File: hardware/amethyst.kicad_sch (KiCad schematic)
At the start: 0 parts

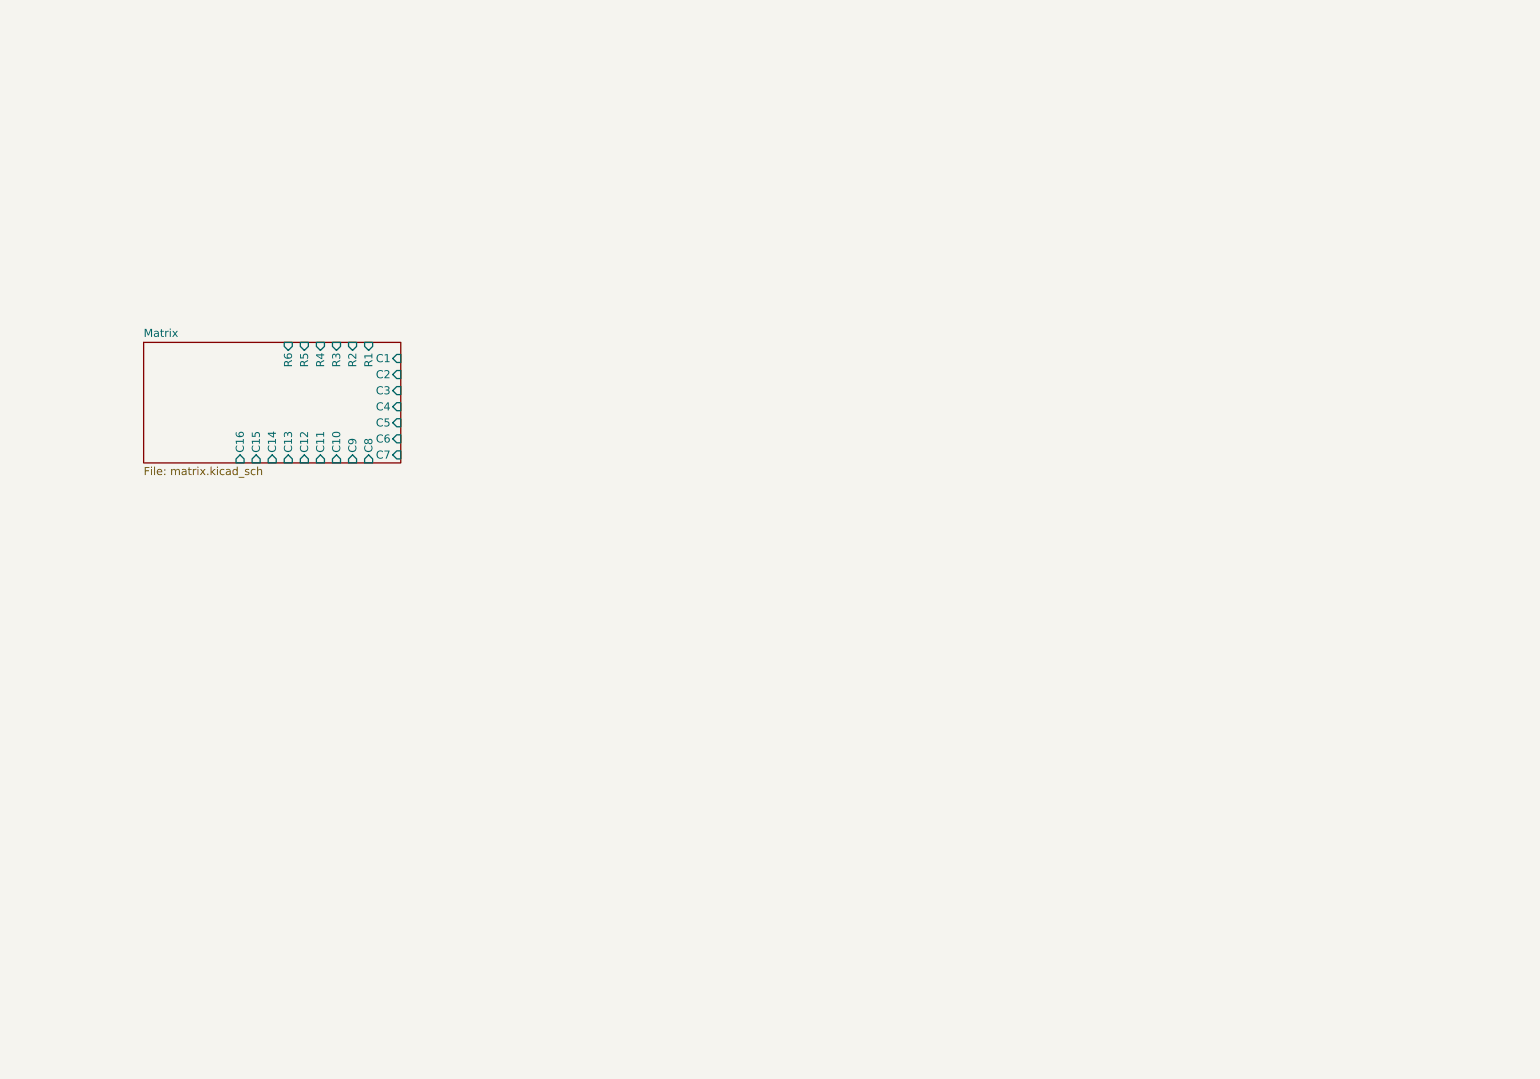
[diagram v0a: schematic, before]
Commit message: Layout done
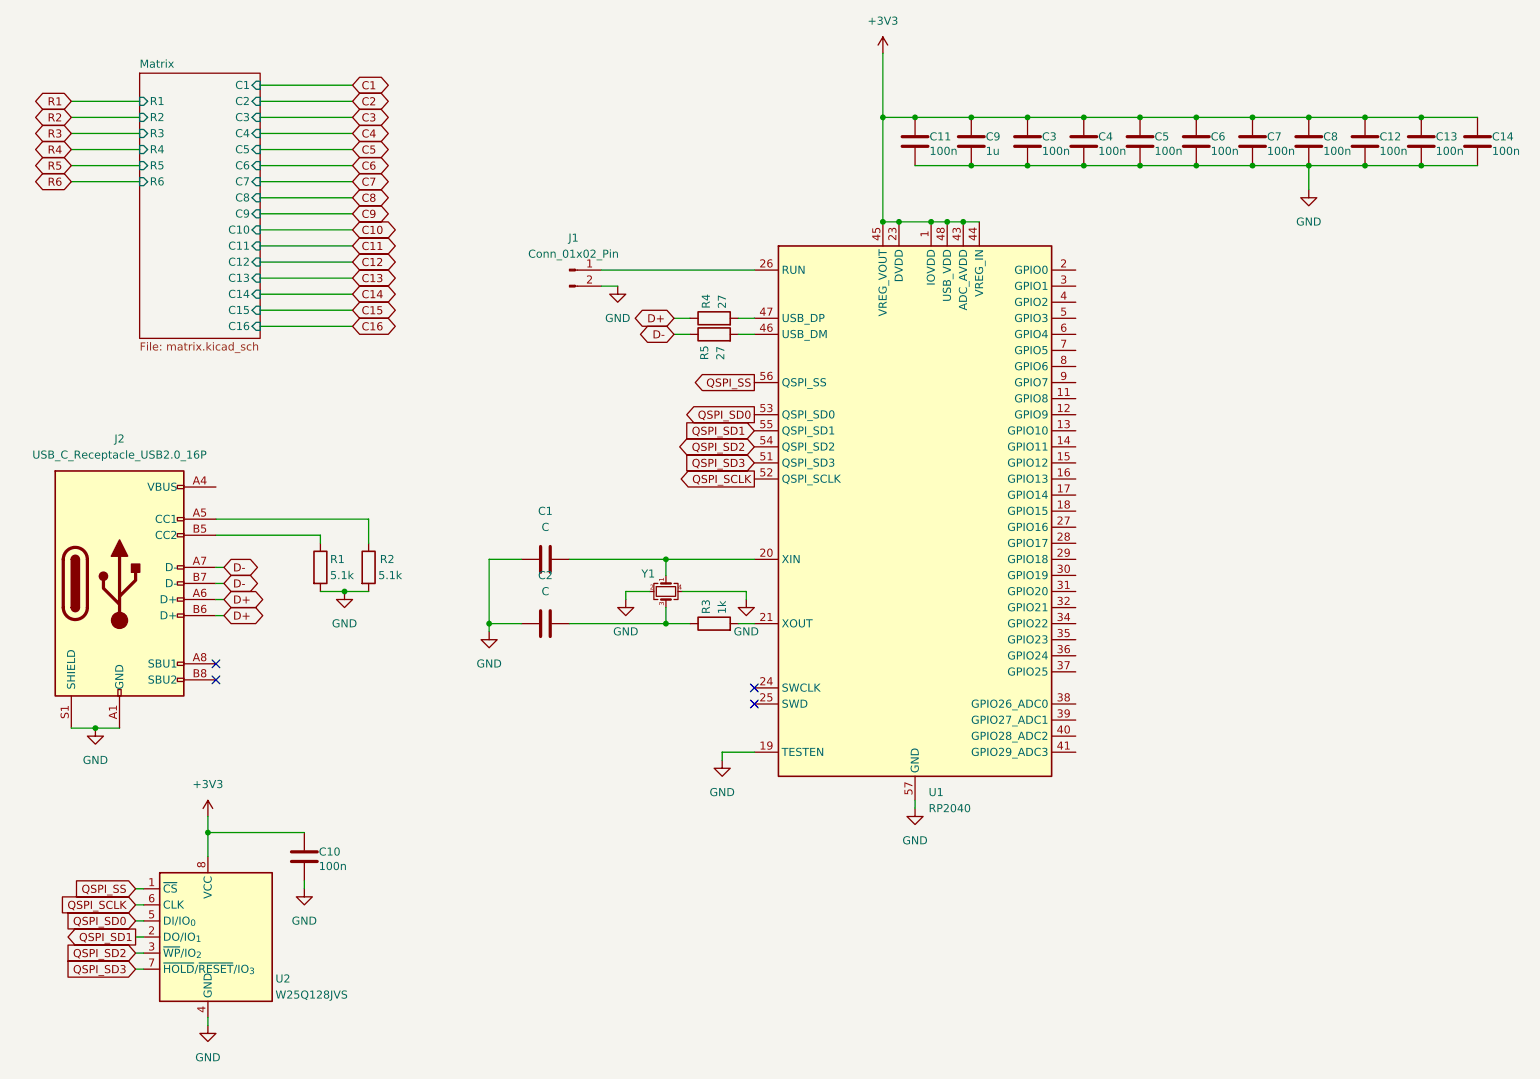
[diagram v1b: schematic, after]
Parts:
- added C1, C2: C, Capacitor_SMD:C_0402_1005Metric, symbol Device:C
- added C10, C11, C12, C13, C14, C3, C4, C5, C6, C7, C8: 100n, Capacitor_SMD:C_0402_1005Metric, symbol Device:C
- added C9: 1u, Capacitor_SMD:C_0402_1005Metric, symbol Device:C
- added J1: Conn_01x02_Pin, Connector_PinHeader_1.00mm:PinHeader_1x02_P1.00mm_Vertical, symbol Connector:Conn_01x02_Pin
- added J2: USB_C_Receptacle_USB2.0_16P, Connector_USB:USB_C_Receptacle_XKB_U262-16XN-4BVC11, symbol Connector:USB_C_Receptacle_USB2.0_16P
- added R1, R2: 5.1k, Resistor_SMD:R_0402_1005Metric, symbol Device:R
- added R3: 1k, Resistor_SMD:R_0402_1005Metric, symbol Device:R
- added R4, R5: 27, Resistor_SMD:R_0402_1005Metric, symbol Device:R
- added U1: RP2040, Package_DFN_QFN:QFN-56-1EP_7x7mm_P0.4mm_EP3.2x3.2mm, symbol MCU_RaspberryPi:RP2040
- added U2: W25Q128JVS, Package_SO:SOIC-8_5.3x5.3mm_P1.27mm, symbol Memory_Flash:W25Q128JVS
- added Y1: Crystal_GND24_Small, Crystal:Crystal_SMD_3225-4Pin_3.2x2.5mm, symbol Device:Crystal_GND24_Small
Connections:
- new net: C2.2, R3.1, Y1.3
- new net: R3.2, U1.21 (XOUT)
- new net: C1.2, U1.20 (XIN), Y1.1
- new net: R4.2, U1.47 (USB_DP)
- new net: J2.A5 (CC1), R2.1
- new net: J2.A4 (VBUS), J2.A9 (VBUS), J2.B4 (VBUS), J2.B9 (VBUS)
- new net: J2.B5 (CC2), R1.1
- new net: J1.1 (Pin_1), U1.26 (RUN)
- new net: R5.2, U1.46 (USB_DM)
- new net +3V3: C10.1, C11.1, C12.1, C13.1, C14.1, C3.1, C4.1, C5.1, C6.1, C7.1, C8.1, C9.1, U1.1 (IOVDD), U1.10 (IOVDD), U1.22 (IOVDD), U1.23 (DVDD), U1.33 (IOVDD), U1.42 (IOVDD), U1.43 (ADC_AVDD), U1.44 (VREG_IN), U1.45 (VREG_VOUT), U1.48 (USB_VDD), U1.49 (IOVDD), U1.50 (DVDD), U2.8 (VCC)
- new net D+: J2.A6 (D+), J2.B6 (D+), R4.1
- new net D-: J2.A7 (D-), J2.B7 (D-), R5.1
- new net GND: C1.1, C10.2, C11.2, C12.2, C13.2, C14.2, C2.1, C3.2, C4.2, C5.2, C6.2, C7.2, C8.2, C9.2, J1.2 (Pin_2), J2.A1 (GND), J2.A12 (GND), J2.B1 (GND), J2.B12 (GND), J2.S1 (SHIELD), R1.2, R2.2, U1.19 (TESTEN), U1.57 (GND), U2.4 (GND), Y1.2, Y1.4
- new net QSPI_SCLK: U1.52 (QSPI_SCLK), U2.6 (CLK)
- new net QSPI_SD0: U1.53 (QSPI_SD0), U2.5 (DI/IO_{0})
- new net QSPI_SD1: U1.55 (QSPI_SD1), U2.2 (DO/IO_{1})
- new net QSPI_SD2: U1.54 (QSPI_SD2), U2.3 (~{WP}/IO_{2})
- new net QSPI_SD3: U1.51 (QSPI_SD3), U2.7 (~{HOLD}/~{RESET}/IO_{3})
- new net QSPI_SS: U1.56 (QSPI_SS), U2.1 (~{CS})
- no-connect marks 0 -> 4
